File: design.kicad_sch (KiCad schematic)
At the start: 181 parts, among them J1 TYPE-C-31-M-12, J301 TYPE-C-31-M-12, U1 TTP223, U10 ATtiny1616-M, U2 TTP223, U3 TTP223, U4 TTP223, U5 TTP223, U6 TTP223, U7 TTP223, U8 TTP223, U9 MAX77751CEFG_T

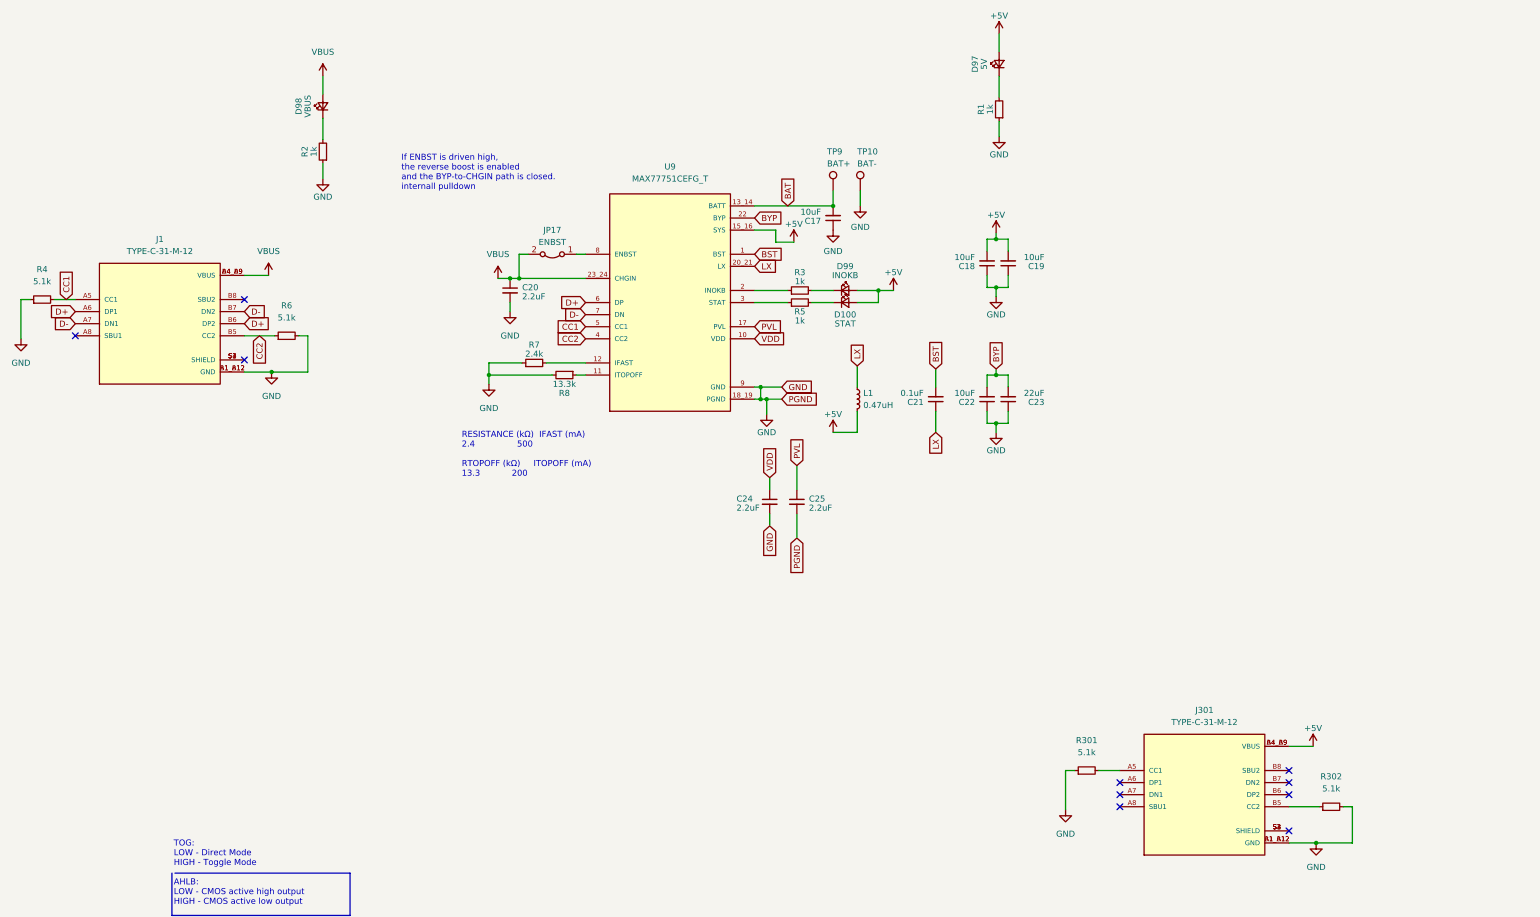
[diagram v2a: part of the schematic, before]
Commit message: upadte
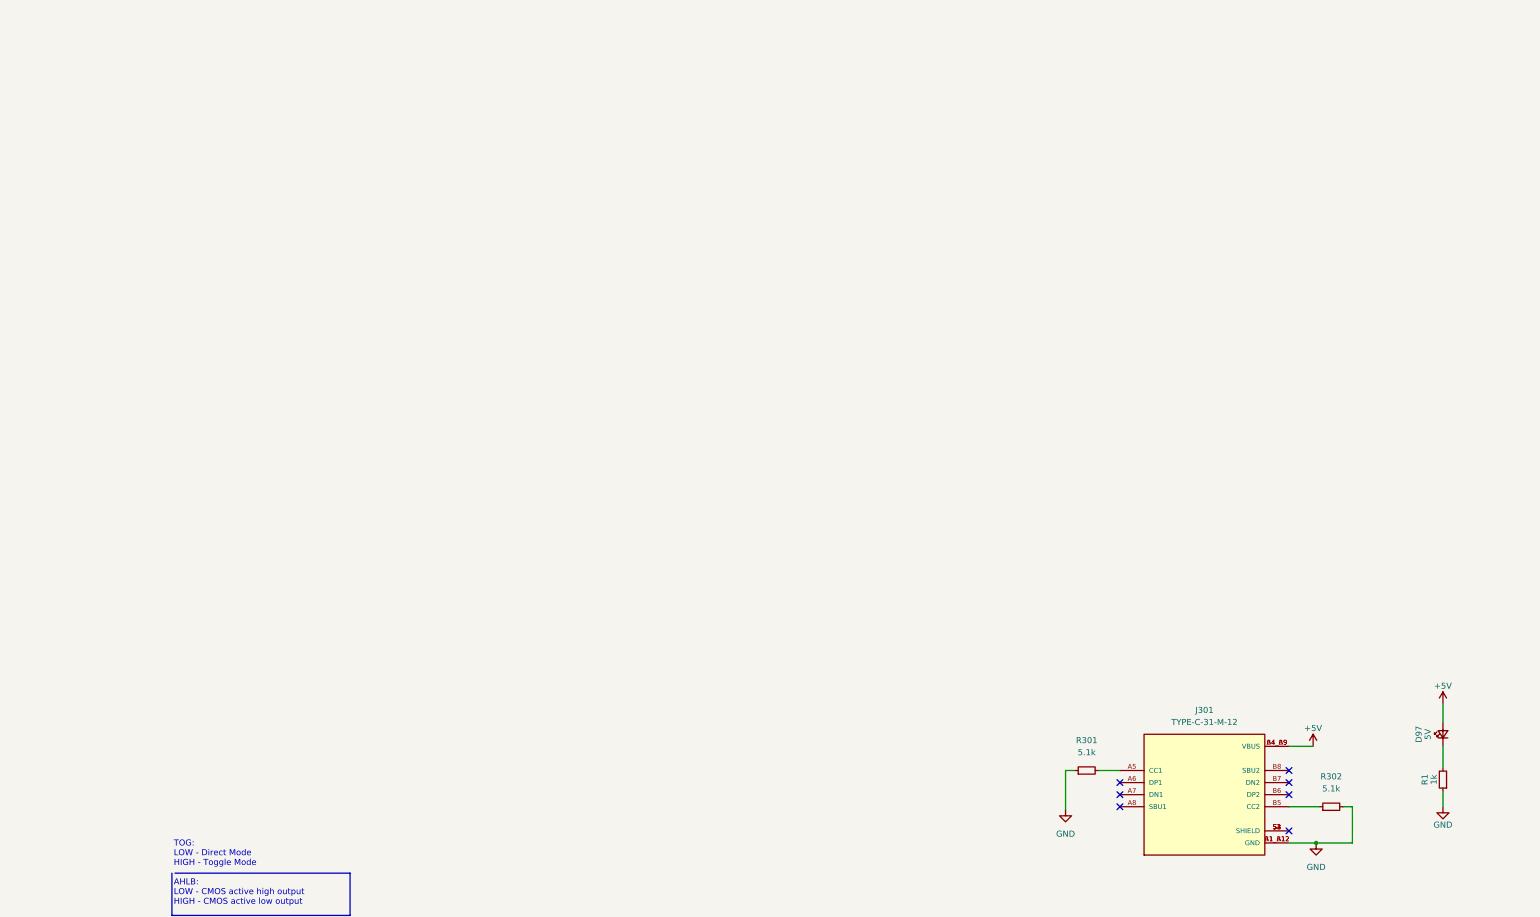
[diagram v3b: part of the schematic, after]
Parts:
- removed C17, C18, C19, C22: 10uF, Capacitor_SMD:C_0805_2012Metric, symbol Device:C_Small
- removed C20, C24, C25: 2.2uF, Capacitor_SMD:C_0805_2012Metric, symbol Device:C_Small
- removed C21: 0.1uF, Capacitor_SMD:C_0805_2012Metric, symbol Device:C_Small
- removed C23: 22uF, Capacitor_SMD:C_0805_2012Metric, symbol Device:C_Small
- removed D100: STAT, LED_SMD:LED_0603_1608Metric, symbol Device:LED_Small
- removed D98: VBUS, LED_SMD:LED_0603_1608Metric, symbol Device:LED_Small
- removed D99: INOKB, LED_SMD:LED_0603_1608Metric, symbol Device:LED_Small
- removed J1: TYPE-C-31-M-12, Snapeda:TYPE-C-31-M-12_HRO_TYPE-C-31-M-12, symbol Snapeda:TYPE-C-31-M-12
- removed JP17: ENBST, LED_SMD:LED_0603_1608Metric, symbol Jumper:Jumper_2_Bridged
- removed L1: 0.47uH, Inductor_SMD:L_0805_2012Metric, symbol Device:L_Small
- removed R2, R3, R5: 1k, Resistor_SMD:R_0805_2012Metric, symbol Device:R_Small
- removed R4, R6: 5.1k, Resistor_SMD:R_0805_2012Metric, symbol Device:R_Small
- removed R7: 2.4k, Resistor_SMD:R_0805_2012Metric, symbol Device:R_Small
- removed R8: 13.3k, Resistor_SMD:R_0805_2012Metric, symbol Device:R_Small
- removed TP10: BAT-, TestPoint:TestPoint_Pad_4.0x4.0mm, symbol Connector:TestPoint
- removed TP9: BAT+, TestPoint:TestPoint_Pad_4.0x4.0mm, symbol Connector:TestPoint
- removed U9: MAX77751CEFG_T, Snapeda:IC_MAX77751CEFG_T, symbol Snapeda:MAX77751CEFG_T
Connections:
- no-connect marks 12 -> 9
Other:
- note removed: "If ENBST is driven high, the reverse boost is enabled and the BYP-to-CHGIN path is closed. internall pulldown"
- note removed: "RESISTANCE (kΩ) IFAST (mA) 2.4 500 RTOPOFF (kΩ) ITOPOFF (mA) 13.3 200"
- moved on the sheet: D97, R1
